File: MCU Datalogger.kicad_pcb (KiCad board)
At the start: 2 copper layers, 45.7 x 30.3 mm, 29 parts, among them J1 Conn_01x04_Pin, J2 Conn_01x09_Pin, J3 Conn_01x04_Pin, J4 Conn_02x03_Odd_Even, U1 24LC1025, U2 24LC1025, U3 DS1337S_, U4 ATMEGA328P-AU, Y1 32.768 KHz, Y2 16 MHz

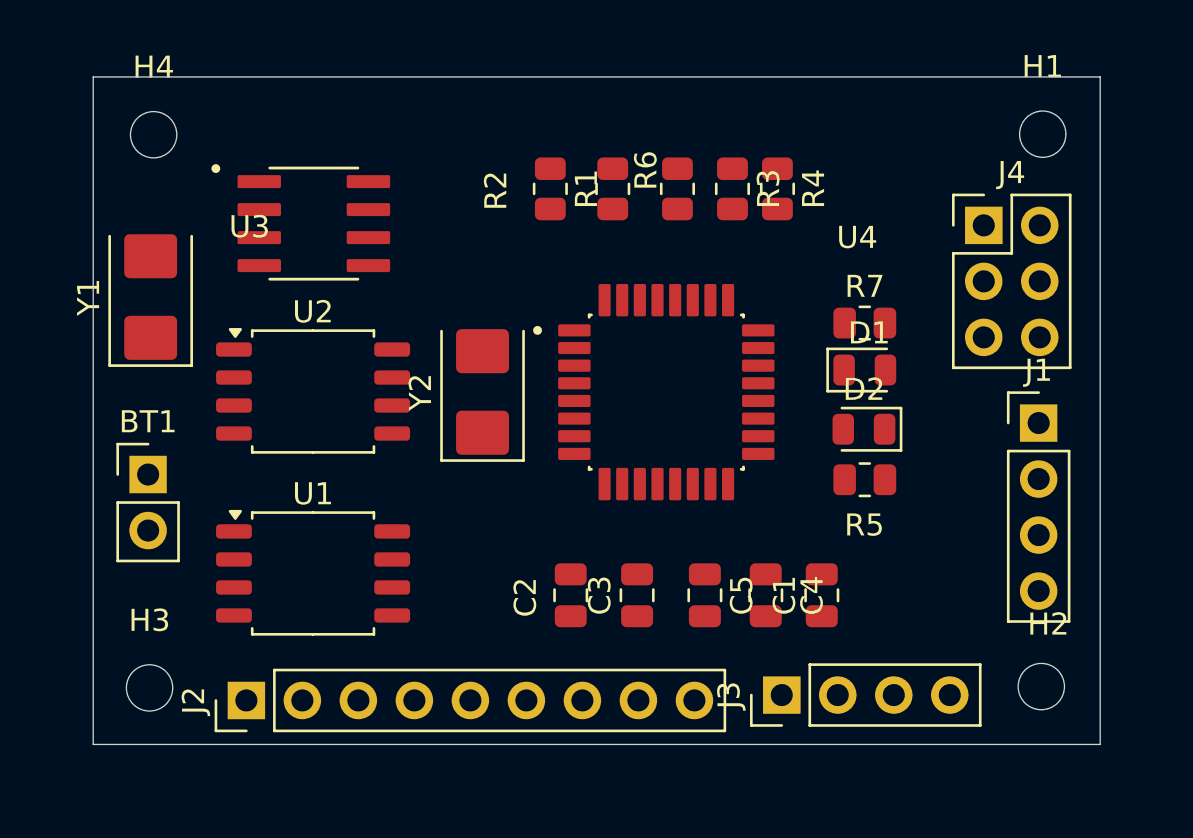
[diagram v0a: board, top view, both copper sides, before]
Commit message: Routing sans GNC VCC complete.
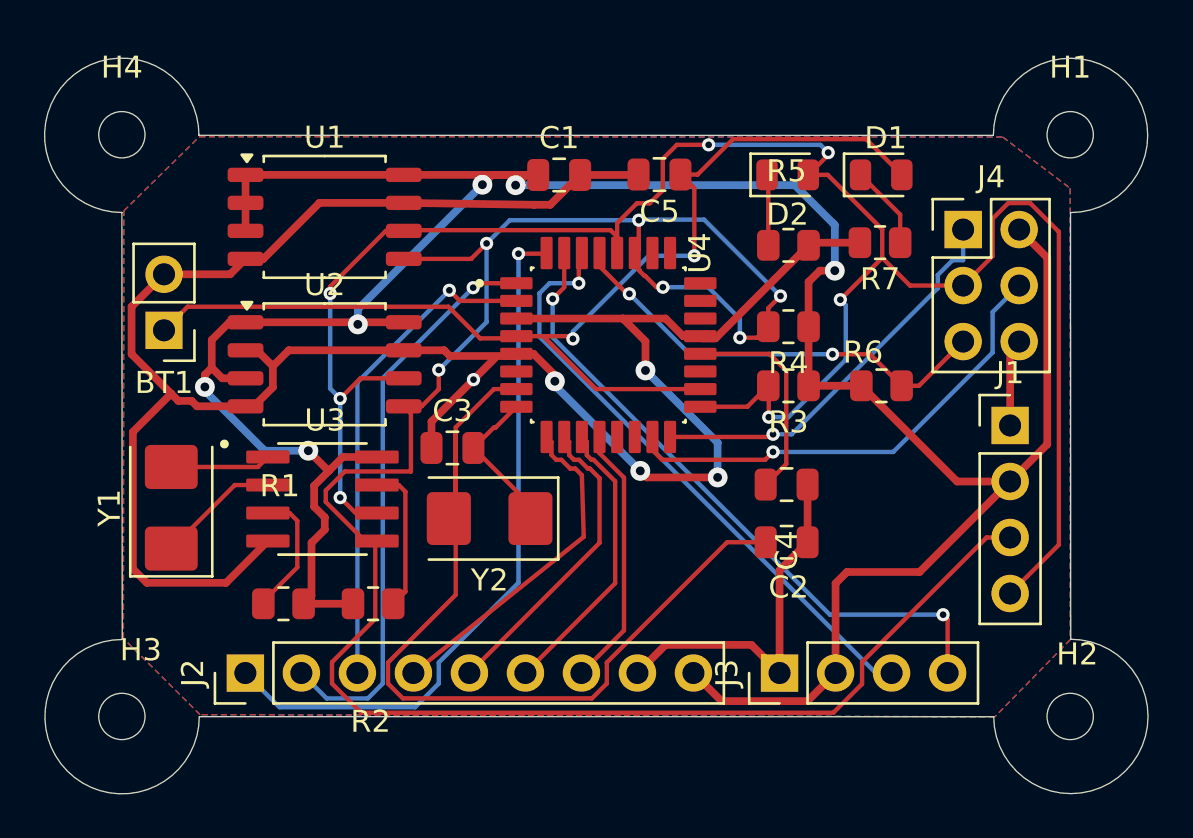
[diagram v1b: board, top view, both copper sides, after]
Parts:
- moved R2 23.3 mm to (121.7, 104.6), turned to 0 degrees
- moved C1 22.5 mm to (130.1, 85.1), turned to 0 degrees
- moved R1 22.4 mm to (117.6, 104.6), turned to 180 degrees
- moved C5 19.2 mm to (134.7, 85.1), turned to 180 degrees
- moved U1 16.2 mm to (119.5, 87.0)
- moved R6 15.1 mm to (144.7, 94.7), turned to 0 degrees
- moved U3 12.5 mm to (119.4, 99.8)
- moved D2 12.0 mm to (140.5, 85.1), turned to 0 degrees
- moved R5 11.2 mm to (140.5, 88.3), turned to 180 degrees
- moved C3 10.7 mm to (125.3, 97.5), turned to 0 degrees
- moved C2 10.1 mm to (140.4, 101.8), turned to 180 degrees
- moved Y1 9.60 mm to (112.5, 100.2)
- moved R3 9.28 mm to (140.5, 94.7), turned to 180 degrees
- moved D1 8.88 mm to (144.7, 85.1)
- moved BT1 6.58 mm to (112.2, 92.2), turned to 180 degrees
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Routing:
- net GND: track 0.00 -> 129.5 mm, vias 0 -> 5
- net /Vcc: track 0.00 -> 128.7 mm, vias 0 -> 6
- net /SCK: track 0.00 -> 94.3 mm, vias 0 -> 7
- net /SDA: track 0.00 -> 94.0 mm, vias 0 -> 6
- net Net-(BT1-+): track 0.00 -> 50.4 mm, vias 0 -> 2
- net Net-(U4-PB6): track 0.00 -> 42.0 mm
- net /D2: track 0.00 -> 32.1 mm, vias 0 -> 1
- net /TX: track 0.00 -> 29.7 mm, vias 0 -> 2
- net /RX: track 0.00 -> 27.7 mm, vias 0 -> 1
- net /D3: track 0.00 -> 26.1 mm, vias 0 -> 1
- net /D4: track 0.00 -> 22.3 mm, vias 0 -> 1
- net /MOSI: track 0.00 -> 21.8 mm, vias 0 -> 1
- net /RESET: track 0.00 -> 20.2 mm, vias 0 -> 2
- net /MISO: track 0.00 -> 18.3 mm, vias 0 -> 1
- net /D5: track 0.00 -> 15.4 mm
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- added copper zone on F.Cu, net /Vcc
- added copper zone on B.Cu, net GND
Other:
- board size 45.7 x 30.3 mm -> 50 x 33.4 mm
